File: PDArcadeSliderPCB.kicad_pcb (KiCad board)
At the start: 2 copper layers, 100 x 63.6 mm, 26 parts, among them J2 Conn_01x06_Male, U1 testsensorg, U2 testsensorg, U3 testsensorg, U4 testsensorg, U5 testsensorg, U6 testsensorg

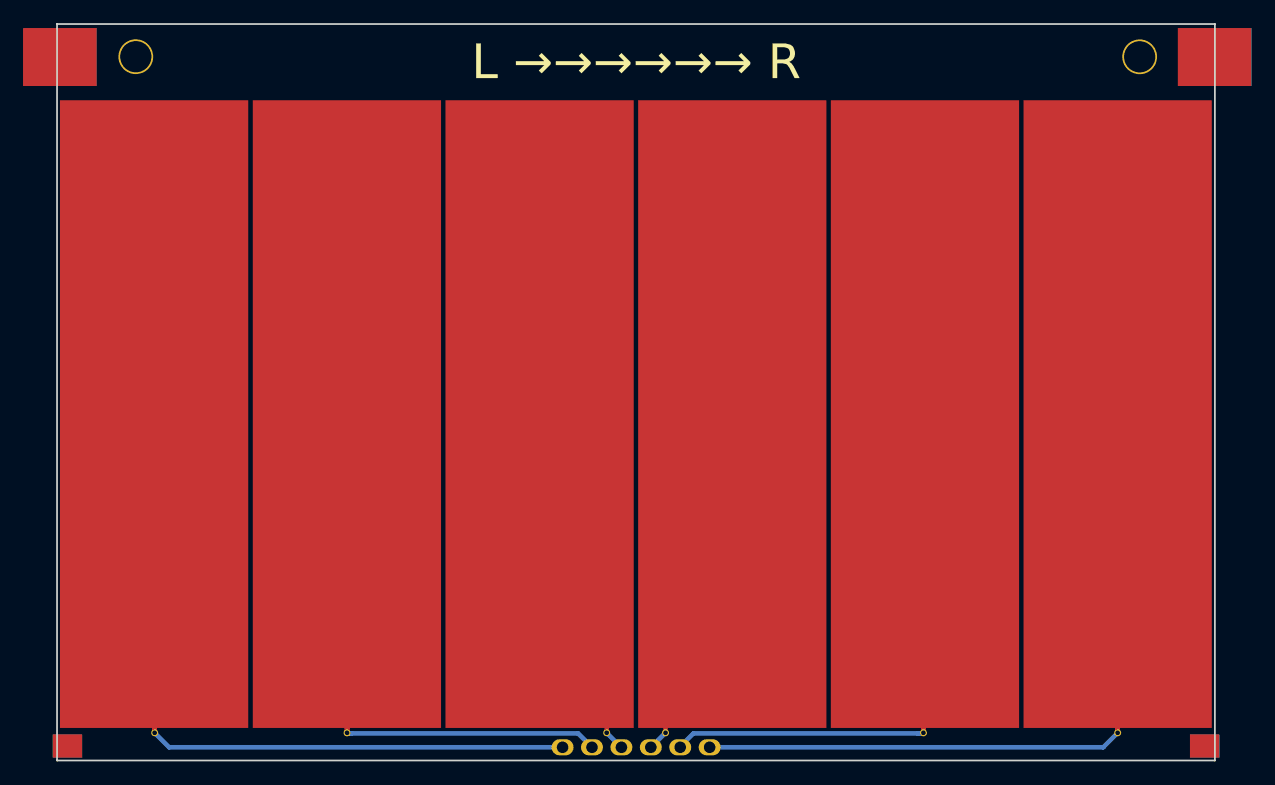
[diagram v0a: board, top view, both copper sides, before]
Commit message: little bigger pads, deleted trash
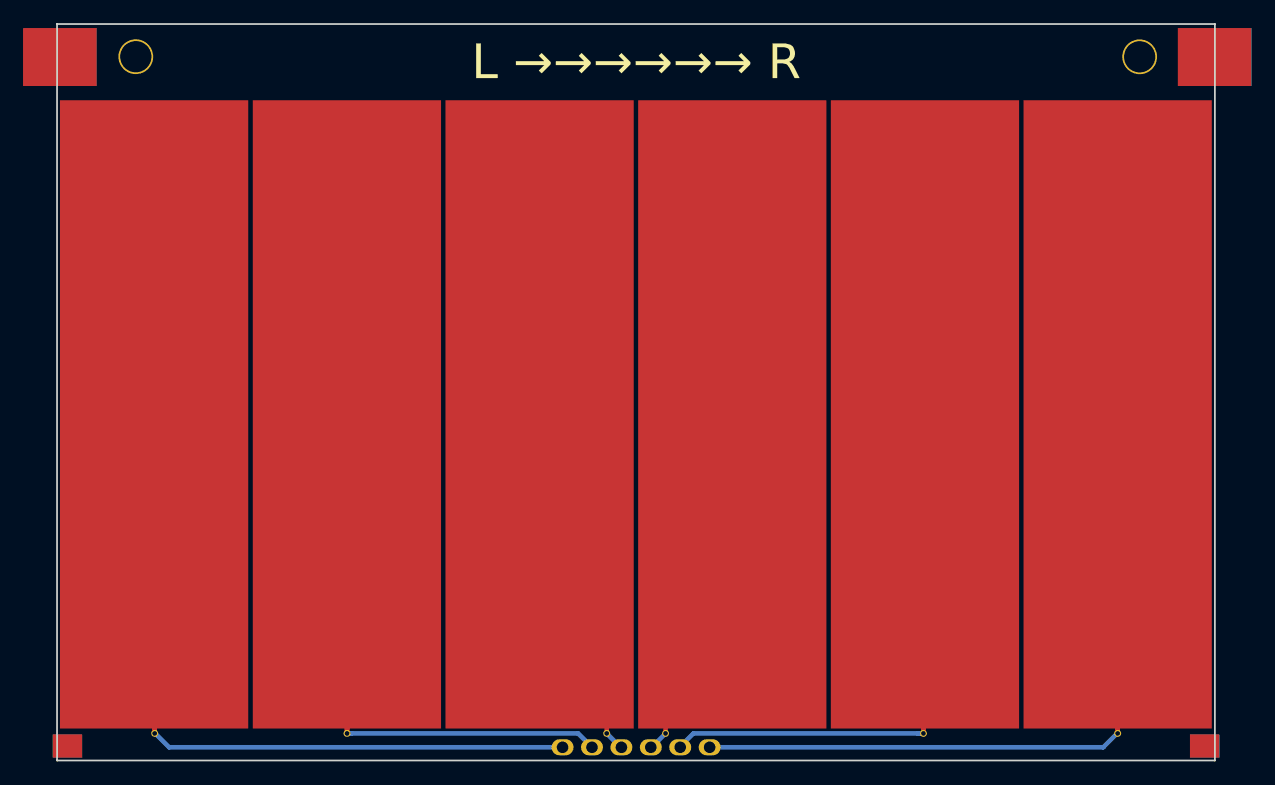
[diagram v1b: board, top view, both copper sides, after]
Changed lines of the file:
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@@
     (thickness 1.6)
     (drawings 7)
-    (tracks 77)
+    (tracks 75)
     (modules 26)
     (nets 8)
@@
       (dimension_precision 1)
     )
-    (pad_size 1.4 1.9)
-    (pad_drill 1)
+    (pad_size 0.6 0.6)
+    (pad_drill 0.4)
     (pad_to_mask_clearance 0.1)
     (solder_mask_min_width 0.15)
@@
     (fp_circle (center 0 0) (end 2.2 0) (layer "Cmts.User") (width 0.15))
     (fp_circle (center 0 0) (end 2.45 0) (layer "F.CrtYd") (width 0.05))
-    (pad "1" thru_hole circle (at 0.22 -5.58 270) (size 0.6 0.6) (drill 0.4) (layers *.Cu *.Mask)
+    (pad "1" thru_hole circle (at 0.27 -5.58 270) (size 0.6 0.6) (drill 0.4) (layers *.Cu *.Mask)
       (net 5 "Net-(J2-Pad4)"))
   )
@@
       (effects (font (size 1 1) (thickness 0.15)))
     )
-    (pad "1" thru_hole circle (at 1.54 0 270) (size 0.6 0.6) (drill 0.4) (layers *.Cu *.Mask)
+    (pad "1" thru_hole circle (at 1.59 0 270) (size 0.6 0.6) (drill 0.4) (layers *.Cu *.Mask)
       (net 1 "Net-(J1-Pad1)"))
   )
@@
     (fp_circle (center 0 0) (end 2.2 0) (layer "Cmts.User") (width 0.15))
     (fp_circle (center 0 0) (end 2.45 0) (layer "F.CrtYd") (width 0.05))
-    (pad "1" thru_hole circle (at 1.52 0 270) (size 0.6 0.6) (drill 0.4) (layers *.Cu *.Mask)
+    (pad "1" thru_hole circle (at 1.57 0 270) (size 0.6 0.6) (drill 0.4) (layers *.Cu *.Mask)
       (net 7 "Net-(J2-Pad2)"))
   )
@@
       (effects (font (size 1 1) (thickness 0.15)))
     )
-    (pad "1" thru_hole circle (at 0.23 5.74 270) (size 0.6 0.6) (drill 0.4) (layers *.Cu *.Mask)
+    (pad "1" thru_hole circle (at 0.28 5.74 270) (size 0.6 0.6) (drill 0.4) (layers *.Cu *.Mask)
       (net 6 "Net-(J2-Pad3)"))
   )
@@
       (effects (font (size 1 1) (thickness 0.15)))
     )
-    (pad "1" thru_hole circle (at 1.49 0 270) (size 0.6 0.6) (drill 0.4) (layers *.Cu *.Mask)
+    (pad "1" thru_hole circle (at 1.54 0 270) (size 0.6 0.6) (drill 0.4) (layers *.Cu *.Mask)
       (net 4 "Net-(J2-Pad5)"))
   )
@@
     (fp_circle (center 0 0) (end 2.2 0) (layer "Cmts.User") (width 0.15))
     (fp_circle (center 0 0) (end 2.45 0) (layer "F.CrtYd") (width 0.05))
-    (pad "1" thru_hole circle (at 1.49 0 270) (size 0.6 0.6) (drill 0.4) (layers *.Cu *.Mask)
+    (pad "1" thru_hole circle (at 1.54 0 270) (size 0.6 0.6) (drill 0.4) (layers *.Cu *.Mask)
       (net 3 "Net-(J2-Pad6)"))
   )
@@
       (effects (font (size 1 1) (thickness 0.15)))
     )
-    (pad "1" connect rect (at -13.15 10.158 270) (size 54.2 16.256) (layers "F.Cu")
+    (pad "1" connect rect (at -13.125 10.158 270) (size 54.25 16.256) (layers "F.Cu")
       (net 1 "Net-(J1-Pad1)"))
   )
@@
       (effects (font (size 1 1) (thickness 0.15)))
     )
-    (pad "1" connect rect (at -13.15 10.16 270) (size 54.2 16.256) (layers "F.Cu")
+    (pad "1" connect rect (at -13.125 10.16 270) (size 54.25 16.256) (layers "F.Cu")
       (net 6 "Net-(J2-Pad3)"))
   )
@@
       (effects (font (size 1 1) (thickness 0.15)))
     )
-    (pad "1" connect rect (at -13.15 10.16 270) (size 54.2 16.256) (layers "F.Cu")
+    (pad "1" connect rect (at -13.125 10.16 270) (size 54.25 16.256) (layers "F.Cu")
       (net 4 "Net-(J2-Pad5)"))
   )
@@
       (effects (font (size 1 1) (thickness 0.15)))
     )
-    (pad "1" connect rect (at -13.15 10.16 270) (size 54.2 16.256) (layers "F.Cu")
+    (pad "1" connect rect (at -13.125 10.16 270) (size 54.25 16.256) (layers "F.Cu")
       (net 7 "Net-(J2-Pad2)"))
   )
@@
       (effects (font (size 1 1) (thickness 0.15)))
     )
-    (pad "1" connect rect (at -13.15 10.16 270) (size 54.2 16.256) (layers "F.Cu")
+    (pad "1" connect rect (at -13.125 10.16 270) (size 54.25 16.256) (layers "F.Cu")
       (net 5 "Net-(J2-Pad4)"))
   )
@@
       (effects (font (size 1 1) (thickness 0.15)))
     )
-    (pad "1" connect rect (at -13.15 10.173 270) (size 54.2 16.256) (layers "F.Cu")
+    (pad "1" connect rect (at -13.125 10.173 270) (size 54.25 16.256) (layers "F.Cu")
       (net 3 "Net-(J2-Pad6)"))
   )
@@
   (gr_line (start 200.075 103.65) (end 200.075 167.24) (layer "Edge.Cuts") (width 0.15))
   (gr_line (start 200.075 167.24) (end 100.1 167.24) (layer "Edge.Cuts") (width 0.15))
+  (segment (start 148.83 166.1) (end 148.76 166.1) (width 0.4) (layer "B.Cu") (net 5))
+  (segment (start 148.76 166.1) (end 147.56 164.9) (width 0.4) (layer "B.Cu") (net 5))
+  (segment (start 151.44 166.1) (end 152.64 164.9) (width 0.4) (layer "B.Cu") (net 6))
   (segment (start 152.64 164.85) (end 152.64 143.094) (width 0.4) (layer "F.Cu") (net 6))
   (segment (start 152.64 143.094) (end 158.404 137.33) (width 0.4) (layer "F.Cu") (net 6))
-  (segment (start 151.37 166.1) (end 151.39 166.1) (width 0.4) (layer "B.Cu") (net 6))
-  (segment (start 151.39 166.1) (end 152.64 164.85) (width 0.4) (layer "B.Cu") (net 6))
   (segment (start 147.56 164.85) (end 147.56 143.123) (width 0.4) (layer "F.Cu") (net 5))
   (segment (start 147.56 143.123) (end 141.767 137.33) (width 0.4) (layer "F.Cu") (net 5))
   (segment (start 148.83 166.1) (end 148.81 166.1) (width 0.4) (layer "B.Cu") (net 5))
-  (segment (start 148.81 166.1) (end 147.56 164.85) (width 0.4) (layer "B.Cu") (net 5))
   (segment (start 191.68 164.7) (end 191.68 164.46) (width 0.4) (layer "F.Cu") (net 1))
   (segment (start 191.68 164.46) (end 191.68 137.25) (width 0.4) (layer "F.Cu") (net 1))
@@
   (segment (start 125.519999 164.899999) (end 145.089999 164.899999) (width 0.4) (layer "B.Cu") (net 4))
   (segment (start 125.189999 164.899999) (end 125.14 164.85) (width 0.4) (layer "B.Cu") (net 4))
-  (segment (start 151.37 166.1) (end 151.38 166.1) (width 0.4) (layer "B.Cu") (net 6))
   (segment (start 156.45 166.1) (end 190.43 166.1) (width 0.4) (layer "B.Cu") (net 1))
   (segment (start 190.43 166.1) (end 191.68 164.85) (width 0.4) (layer "B.Cu") (net 1))
@@
   (segment (start 153.91 166.1) (end 153.91 166.04) (width 0.4) (layer "B.Cu") (net 7))
   (segment (start 153.91 166.04) (end 155.050001 164.899999) (width 0.4) (layer "B.Cu") (net 7))
-  (segment (start 151.32 166.1) (end 151.32 166.01) (width 0.4) (layer "B.Cu") (net 6))
   (segment (start 174.909 135.372) (end 175.041 135.24) (width 0.4) (layer "F.Cu") (net 7))
   (segment (start 175.036 135.245) (end 175.041 135.24) (width 0.4) (layer "F.Cu") (net 7))
